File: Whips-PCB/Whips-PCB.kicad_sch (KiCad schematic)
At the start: 5 parts, among them SW1 SW_DIP_x05, U1 Teensy4.0, U2 MAX485E, U3 SN74AHCT125, U4 TSR_1-2450

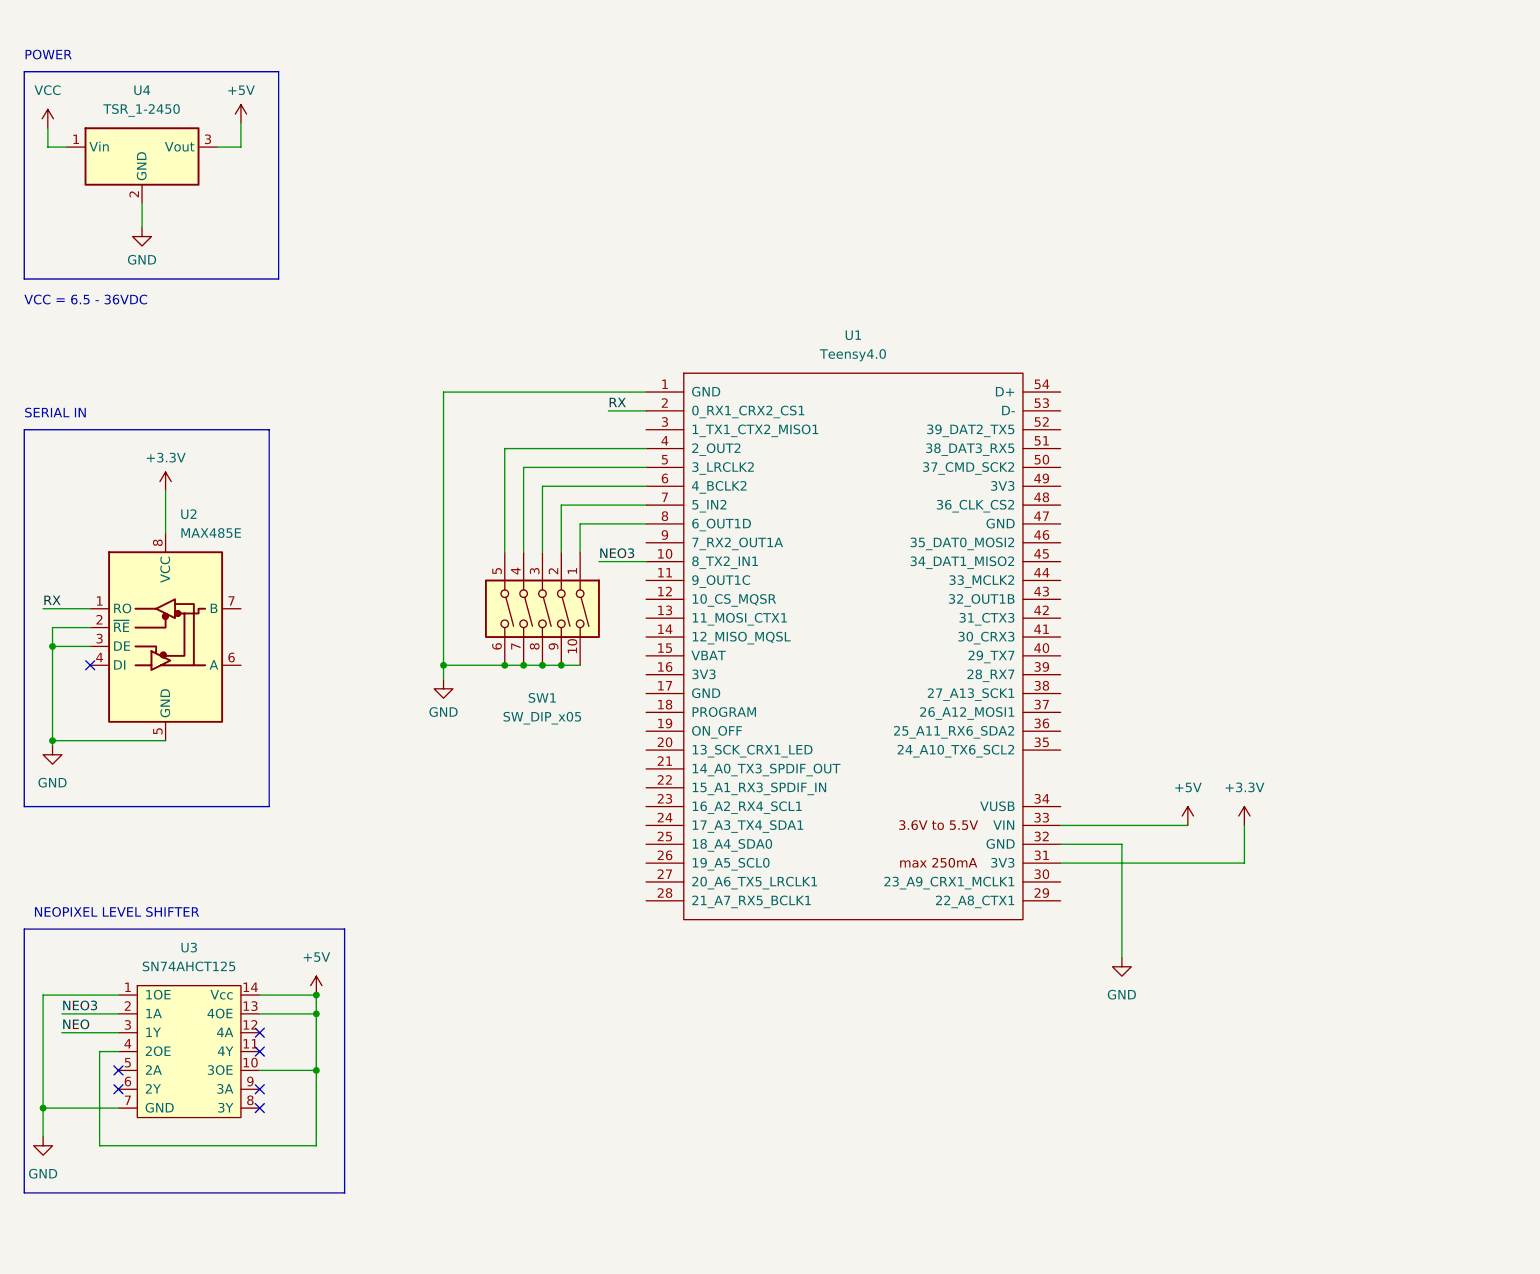
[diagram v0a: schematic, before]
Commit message: improved rs422
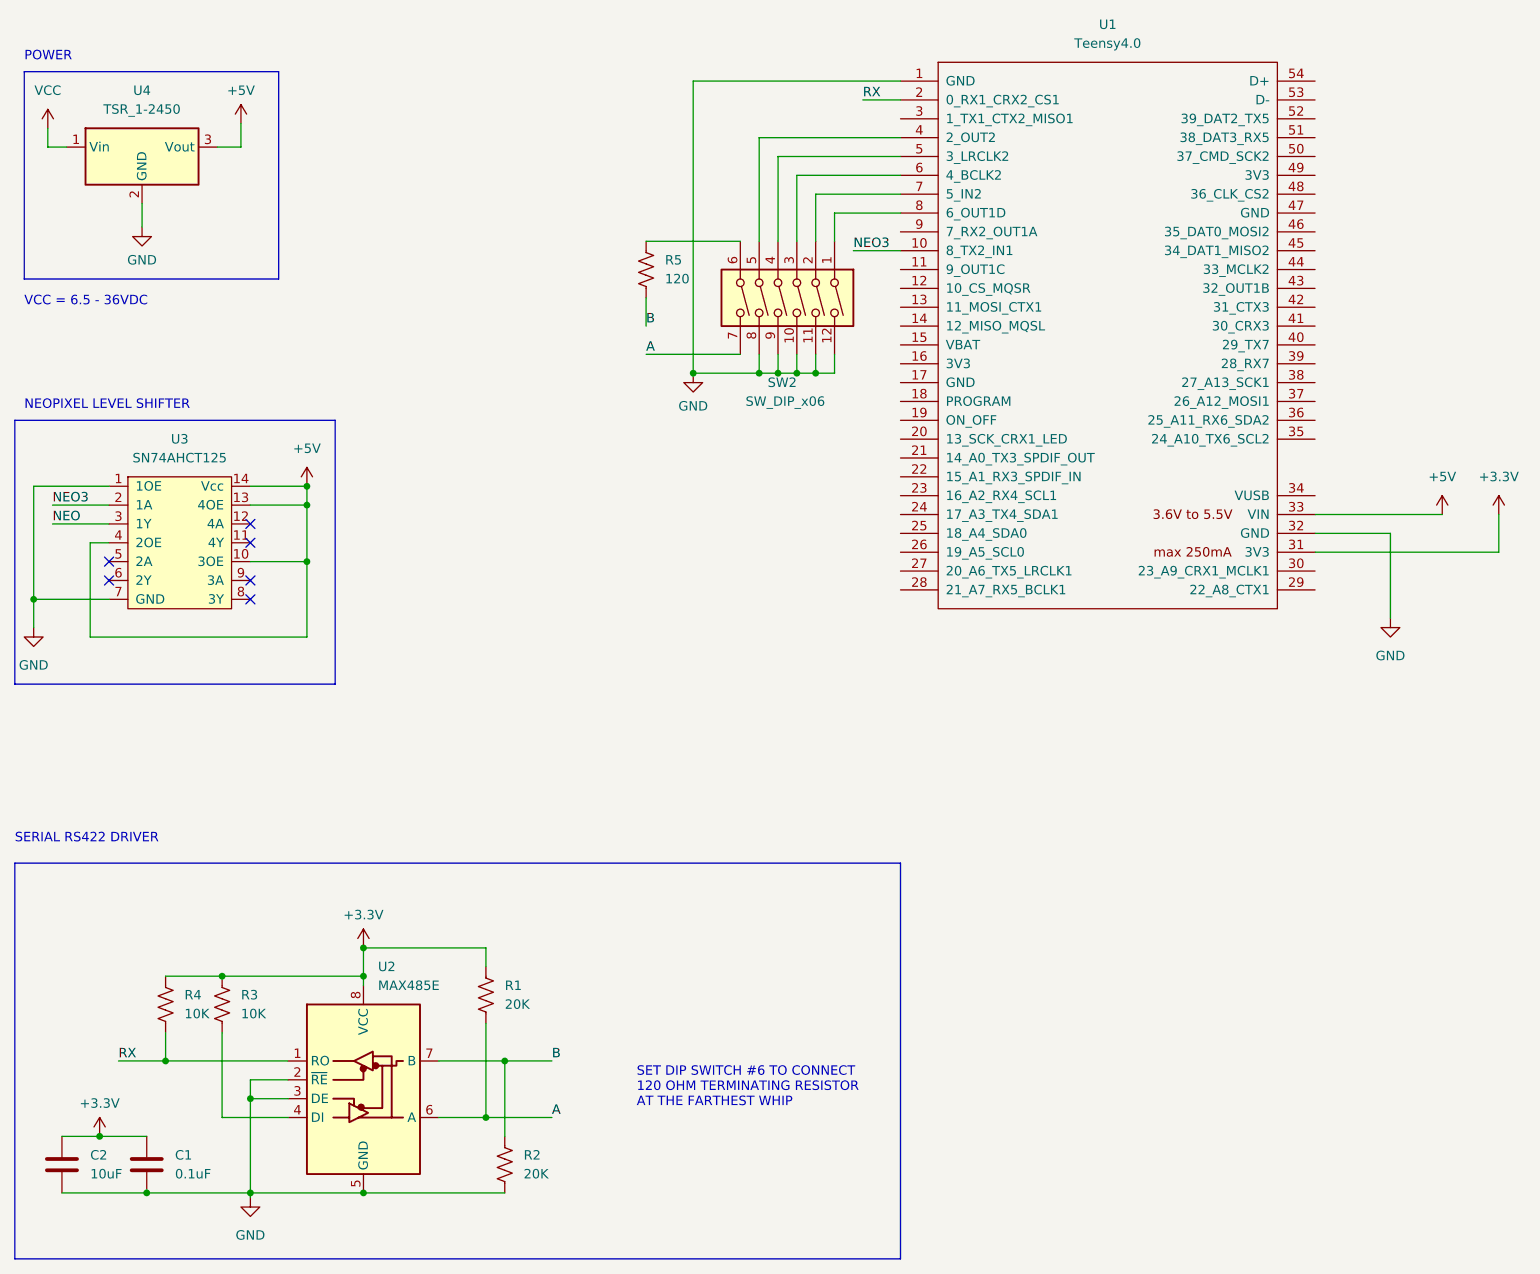
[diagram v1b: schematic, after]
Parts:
- removed SW1: SW_DIP_x05, symbol Switch:SW_DIP_x05
- added C1: 0.1uF, symbol Device:C
- added C2: 10uF, symbol Device:C
- added R1, R2: 20K, symbol Device:R_US
- added R3, R4: 10K, symbol Device:R_US
- added R5: 120, symbol Device:R_US
- added SW2: SW_DIP_x06, symbol Switch:SW_DIP_x06
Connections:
- net +3.3V: now also C1.1, C2.1, R1.1, R3.1, R4.1
- net GND: now also C1.2, C2.2, R2.2, SW2.10, SW2.11, SW2.12, SW2.8, SW2.9
- net RX: now also R4.2
- net at U1.4 (2_OUT2): now also SW2.5
- net at U1.5 (3_LRCLK2): now also SW2.4
- net at U1.6 (4_BCLK2): now also SW2.3
- net at U1.7 (5_IN2): now also SW2.2
- net at U1.8 (6_OUT1D): now also SW2.1
- net at U2.4 (DI): now also R3.2
- net A: now reaches U2.6 (A)
- net A: now also R1.2, SW2.7
- net B: now reaches U2.7 (B)
- net B: now also R2.1, R5.2
- new net: R5.1, SW2.6
- no-connect marks 7 -> 6
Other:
- note added: "SERIAL RS422 DRIVER"
- note added: "SET DIP SWITCH #6 TO CONNECT 120 OHM TERMINATING RESISTOR AT THE FARTHEST WHIP"
- note removed: "SERIAL IN"
- moved on the sheet: U1, U2, U3
